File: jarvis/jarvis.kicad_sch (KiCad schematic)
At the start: 37 parts, among them IC1 ESP32-S3R16V, IC2 MAX98357AETE+T, IC3 MCP73871T-4CAI_ML, IC4 TLV70033DDCT, J1 Conn_01x02 - Speaker, J2 Mic Conn_01x05, J3 Conn_01x02 - Battery, U1 W25Q64JVSSIQ, U2 2137160001, Y1 Crystal 32.768khz, Y2 Crystal 40mhz

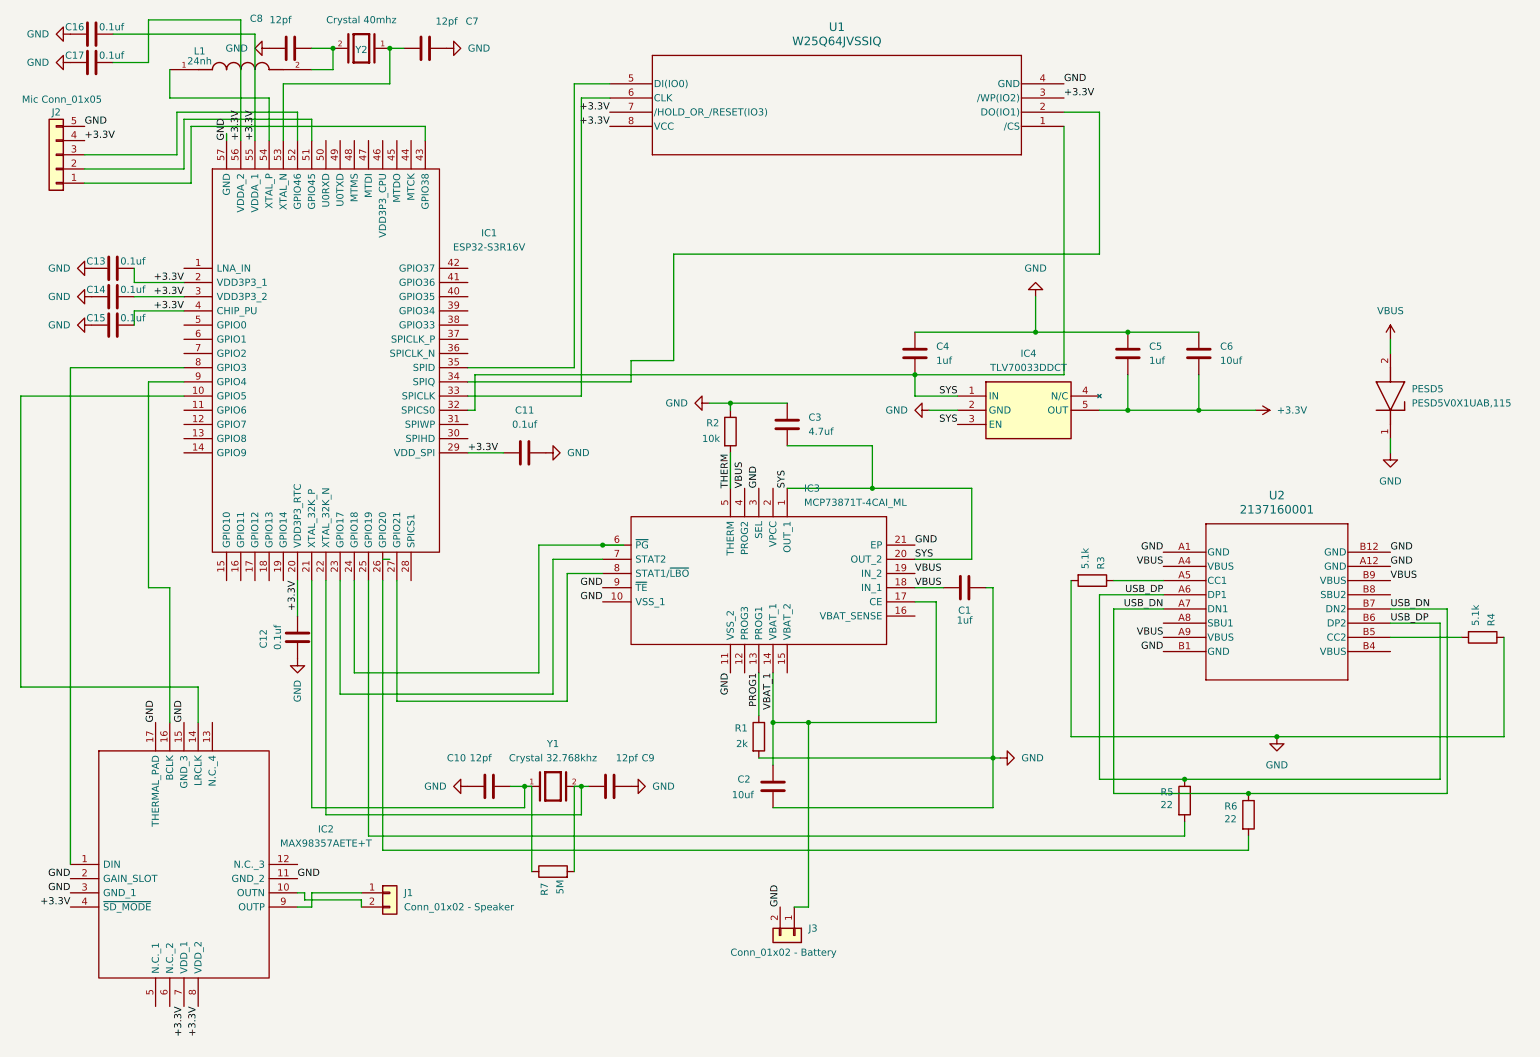
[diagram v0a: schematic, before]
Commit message: flash routed
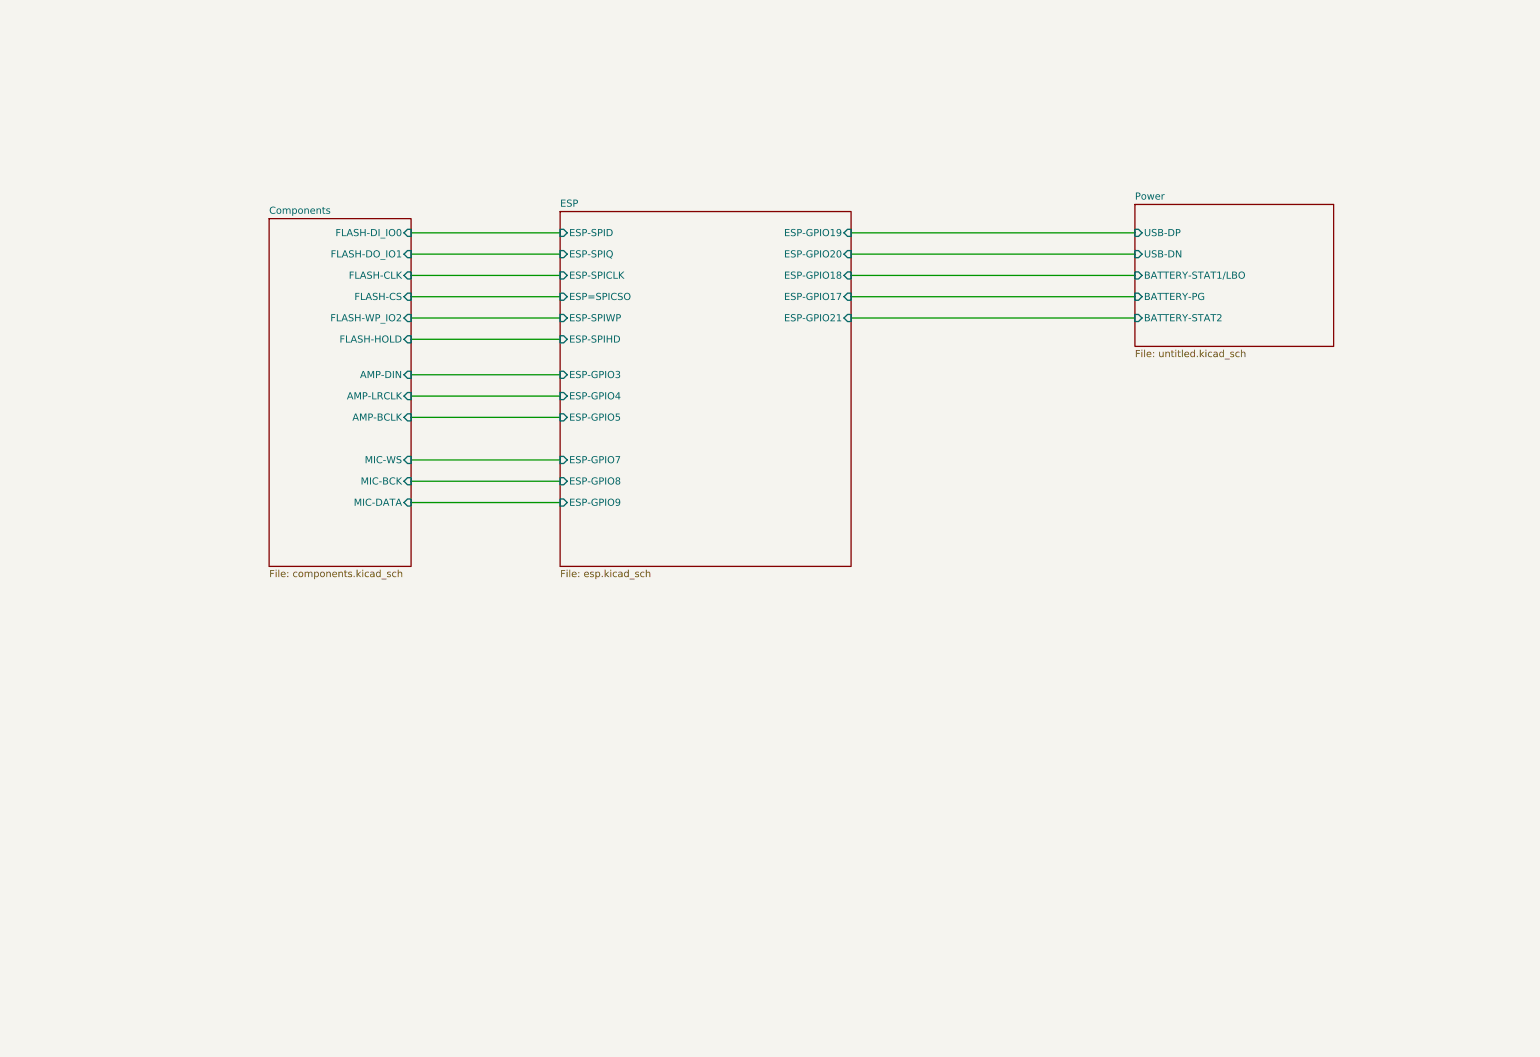
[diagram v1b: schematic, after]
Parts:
- removed C1, C4, C5: 1uf, Capacitor_SMD:C_0603_1608Metric, symbol Device:C
- removed C10, C7, C8, C9: 12pf, Capacitor_SMD:C_0402_1005Metric, symbol Device:C
- removed C11, C12, C13, C14, C15, C16, C17: 0.1uf, Capacitor_SMD:C_0603_1608Metric, symbol Device:C
- removed C2, C6: 10uf, Capacitor_SMD:C_0603_1608Metric, symbol Device:C
- removed C3: 4.7uf, Capacitor_SMD:C_0603_1608Metric, symbol Device:C
- removed IC1: ESP32-S3R16V, jarvis:esp32-s3r16v, symbol jarvis:ESP32-S3R16V
- removed IC2: MAX98357AETE+T, jarvis:LIB_MAX98357AETE+T, symbol jarvis:MAX98357AETE+T
- removed IC3: MCP73871T-4CAI_ML, jarvis:MCP73871T-4CAI ML, symbol jarvis:MCP73871T-4CAI_ML
- removed IC4: TLV70033DDCT, jarvis:TLV70033DDCT, symbol jarvis:TLV70033DDCT
- removed J1: Conn_01x02 - Speaker, Connector_Molex:Molex_PicoBlade_53047-0210_1x02_P1.25mm_Vertical, symbol Connector_Generic:Conn_01x02
- removed J2: Mic Conn_01x05, Connector_Molex:Molex_PicoBlade_53047-0510_1x05_P1.25mm_Vertical, symbol Connector_Generic:Conn_01x05
- removed J3: Conn_01x02 - Battery, Connector_Molex:Molex_PicoBlade_53047-0210_1x02_P1.25mm_Vertical, symbol Connector_Generic:Conn_01x02
- removed L1: 24nh, jarvis:MLG1005SR24JT000, symbol jarvis:MLG1005SR24JT000
- removed PESD5: PESD5V0X1UAB,115, jarvis:PESD5V0X1UAB115, symbol jarvis:PESD5V0X1UAB,115
- removed R1: 2k, Resistor_SMD:R_0603_1608Metric, symbol Device:R
- removed R2: 10k, Resistor_SMD:R_0603_1608Metric, symbol Device:R
- removed R3, R4: 5.1k, Resistor_SMD:R_0603_1608Metric, symbol Device:R
- removed R5, R6: 22, Resistor_SMD:R_0603_1608Metric, symbol Device:R
- removed R7: 5M, Resistor_SMD:R_0603_1608Metric, symbol Device:R
- removed U1: W25Q64JVSSIQ, jarvis:W25Q64JVSSIQ, symbol jarvis:W25Q64JVSSIQ
- removed U2: 2137160001, jarvis:2137160001_MOL, symbol jarvis:2137160001
- removed Y1: Crystal 32.768khz, jarvis:XTAL_CM8V-T1A-32.768KHZ-7PF-20PPM-TA-QC, symbol jarvis:CM8V-T1A-32.768KHZ-7PF-20PPM-TA-QC
- removed Y2: Crystal 40mhz, jarvis:XTAL_CM8V-T1A-32.768KHZ-7PF-20PPM-TA-QC, symbol jarvis:CM8V-T1A-32.768KHZ-7PF-20PPM-TA-QC
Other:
- added sheet Components (components.kicad_sch)
- added sheet ESP (esp.kicad_sch)
- added sheet Power (untitled.kicad_sch)
